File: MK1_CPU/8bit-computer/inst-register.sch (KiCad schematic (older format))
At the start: 28 parts, among them U58 74HCT08, U60 74HCT245, U61 74HCT273, U62 74HCT273, U63 74HCT04

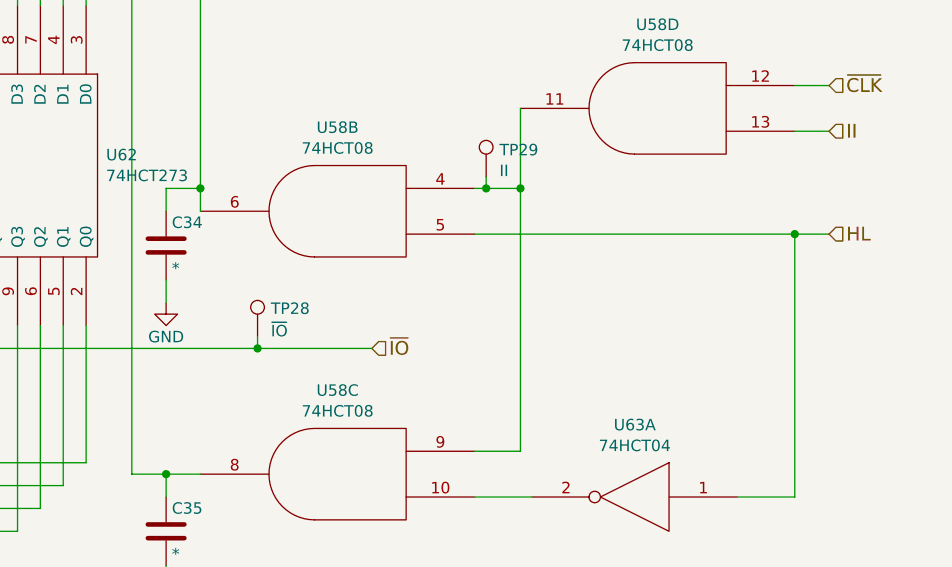
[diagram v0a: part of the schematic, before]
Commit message: 2.0b hardware revision
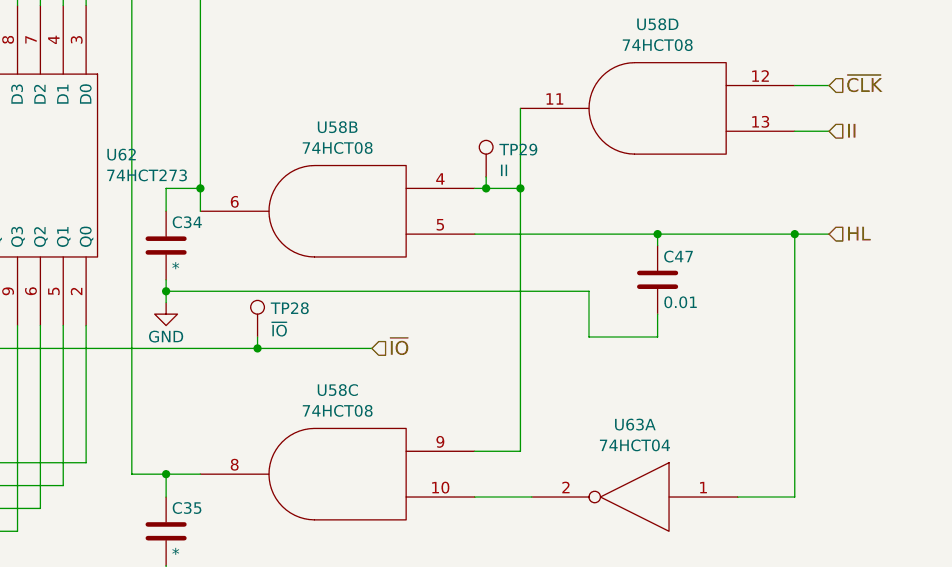
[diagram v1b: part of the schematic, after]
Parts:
- added C47: 0.01, Capacitor_THT:C_Disc_D4.3mm_W1.9mm_P5.00mm, symbol Device:C
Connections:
- net GND: now also C47.2
- net HL: now also C47.1
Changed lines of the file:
@@
 	10000 2600 10150 2600
 Wire Wire Line
-	8600 3050 10000 3050
+	8600 3050 9400 3050
 Wire Wire Line
 	7400 1800 7400 2850
 Wire Wire Line
 	10000 3050 10000 4200
-Connection ~ 10000 3050
-Wire Wire Line
-	10000 3050 10150 3050
 Wire Wire Line
 	7100 2000 7100 4100
@@
 $EndComp
 Wire Wire Line
-	7250 3250 7250 3350
+	7250 3250 7250 3300
 Wire Wire Line
 	7250 2950 7250 2850
@@
 Wire Wire Line
 	1950 3250 1950 4750
+Connection ~ 10000 3050
+Wire Wire Line
+	10000 3050 10150 3050
+$Comp
+L Device:C C47
+U 1 1 5F13FC24
+P 9400 3250
+F 0 "C47" H 9425 3350 50  0000 L CNN
+F 1 "0.01" H 9425 3150 50  0000 L CNN
+F 2 "Capacitor_THT:C_Disc_D4.3mm_W1.9mm_P5.00mm" H 9438 3100 50  0001 C CNN
+F 3 "" H 9400 3250 50  0001 C CNN
+	1    9400 3250
+	1    0    0    -1
+$EndComp
+Wire Wire Line
+	9400 3400 9400 3500
+Wire Wire Line
+	9400 3100 9400 3050
+Connection ~ 9400 3050
+Wire Wire Line
+	9400 3050 10000 3050
+Wire Wire Line
+	7250 3300 9100 3300
+Wire Wire Line
+	9100 3300 9100 3500
+Wire Wire Line
+	9100 3500 9400 3500
+Connection ~ 7250 3300
+Wire Wire Line
+	7250 3300 7250 3350
 $EndSCHEMATC
